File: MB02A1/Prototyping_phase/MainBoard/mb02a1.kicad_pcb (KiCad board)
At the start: 2 copper layers, 7.3 x 1.2 mm, 74 parts, among them J1 USB B mini, J2 USB B mini, J3 USB B mini, J4 USB B mini, U1 CH340G, U11 ACS712-05B, U13 DS1307Z+, U2 CH340G, U3 CH340G, U4 AMS1117-3.3, U5 W25Q64JVS, U6 25LC256, U7 25LC640, U8 NUCLEO-F446RE, U9 WEMOS_D1_mini, X1 12MHz, X2 12MHz, X3 12MHz, X4 32.768 kHz

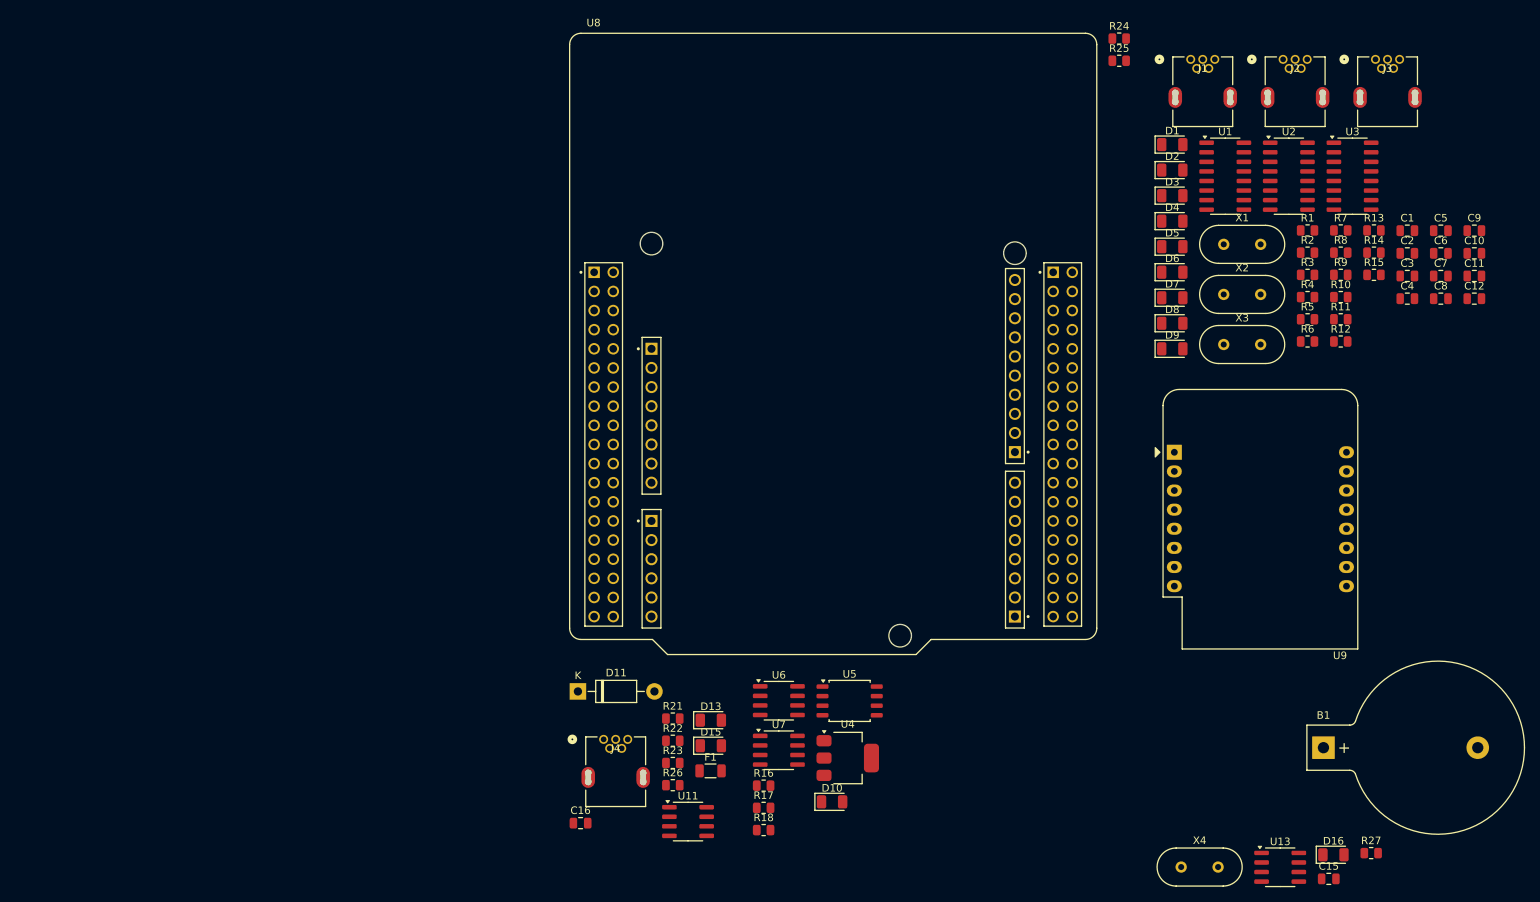
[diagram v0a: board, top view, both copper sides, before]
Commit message: Design update, production preparation.
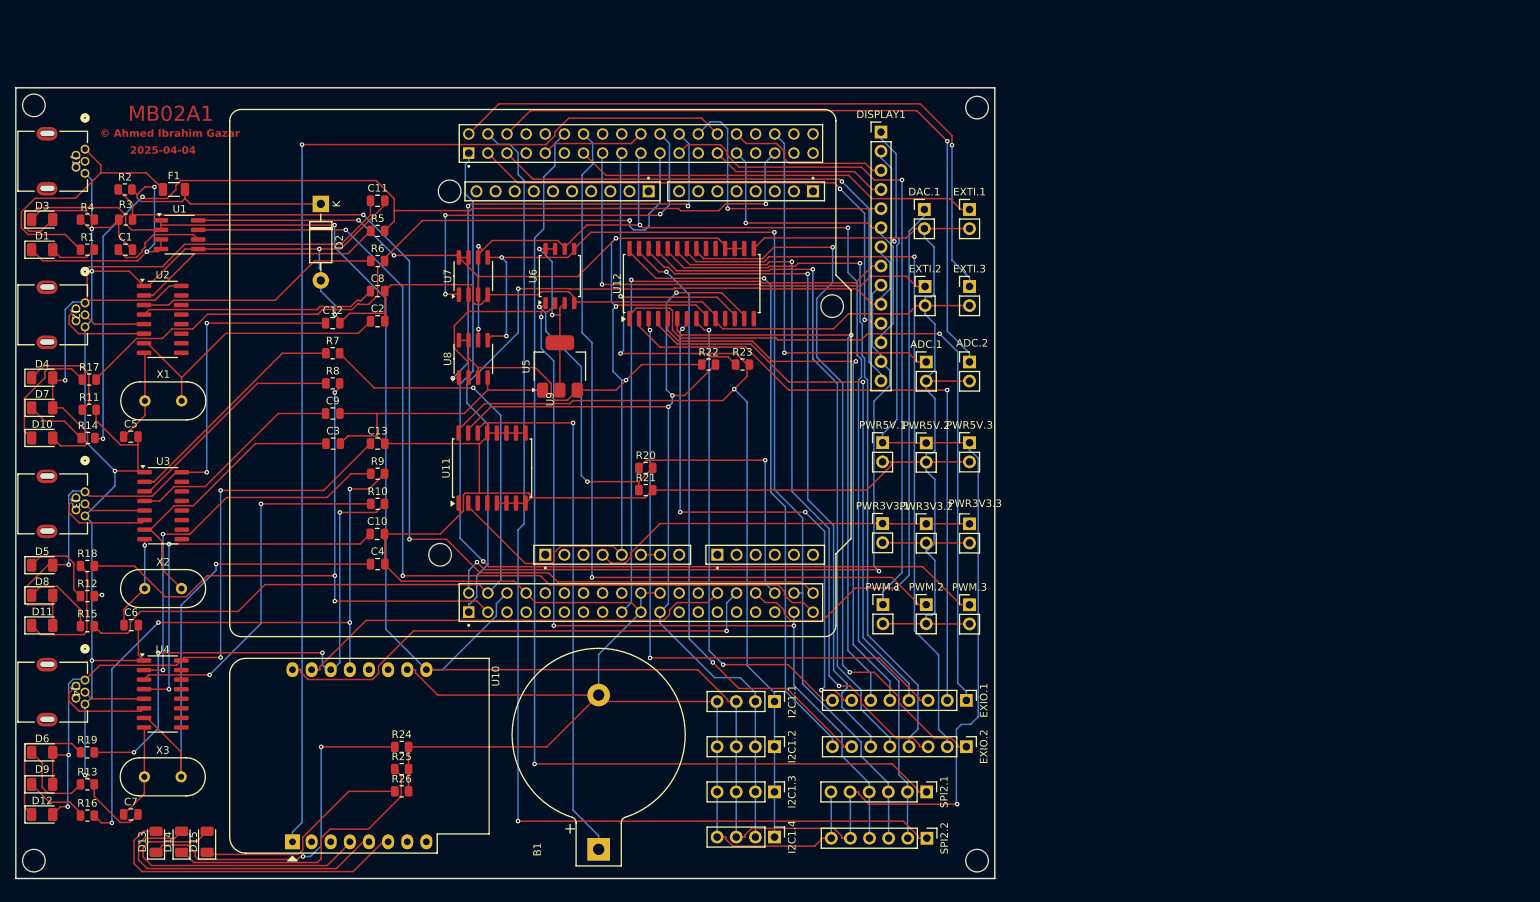
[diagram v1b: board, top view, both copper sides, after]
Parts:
- removed C15: 100p, Capacitor_SMD:C_0805_2012Metric
- removed C16: 1n, Capacitor_SMD:C_0805_2012Metric
- removed D16: D_Schottky, Diode_SMD:D_1206_3216Metric
- removed R27: 1k, Resistor_SMD:R_0805_2012Metric
- removed U13: DS1307Z+, Package_SO:SOIC-8_3.9x4.9mm_P1.27mm
- removed X4: 32.768 kHz, Crystal:Crystal_HC18-U_Vertical
- added ?: , , F.Cu at (80.5, 49.7)
- added ?: , , F.Cu at (80.5, 150.0)
- added ?: , , F.Cu at (205.8, 150.0)
- added ?: , , F.Cu at (205.8, 50.0)
- added ADC.1: Conn_01x02_Pin, Connector_PinHeader_2.54mm:PinHeader_1x02_P2.54mm_Vertical, F.Cu at (199.0, 83.8)
- added ADC.2: Conn_01x02_Pin, Connector_PinHeader_2.54mm:PinHeader_1x02_P2.54mm_Vertical, F.Cu at (204.8, 83.8)
- added C13: 100n, Capacitor_SMD:C_0805_2012Metric, F.Cu at (126.2, 94.6)
- added D12: LED, LED_SMD:LED_1206_3216Metric, F.Cu at (81.6, 143.9)
- added D14: LED, LED_SMD:LED_1206_3216Metric, F.Cu at (100.1, 147.5)
- added DAC.1: Conn_01x02_Pin, Connector_PinHeader_2.54mm:PinHeader_1x02_P2.54mm_Vertical, F.Cu at (198.8, 63.5)
- added DISPLAY1: Conn_01x14_Pin, Connector_PinHeader_2.54mm:PinHeader_1x14_P2.54mm_Vertical, F.Cu at (193.0, 53.3)
- added EXIO.1: Conn_01x08_Pin, Connector_PinHeader_2.54mm:PinHeader_1x08_P2.54mm_Vertical, F.Cu at (204.3, 128.7)
- added EXIO.2: Conn_01x08_Pin, Connector_PinHeader_2.54mm:PinHeader_1x08_P2.54mm_Vertical, F.Cu at (204.3, 134.9)
- added EXTI.1: Conn_01x02_Pin, Connector_PinHeader_2.54mm:PinHeader_1x02_P2.54mm_Vertical, F.Cu at (204.8, 63.5)
- added EXTI.2: Conn_01x02_Pin, Connector_PinHeader_2.54mm:PinHeader_1x02_P2.54mm_Vertical, F.Cu at (198.8, 73.8)
- added EXTI.3: Conn_01x02_Pin, Connector_PinHeader_2.54mm:PinHeader_1x02_P2.54mm_Vertical, F.Cu at (204.8, 73.8)
- added I2C1.1: Conn_01x04_Pin, Connector_PinHeader_2.54mm:PinHeader_1x04_P2.54mm_Vertical, F.Cu at (178.8, 128.9)
- added I2C1.2: Conn_01x04_Pin, Connector_PinHeader_2.54mm:PinHeader_1x04_P2.54mm_Vertical, F.Cu at (178.8, 134.9)
- added I2C1.3: Conn_01x04_Pin, Connector_PinHeader_2.54mm:PinHeader_1x04_P2.54mm_Vertical, F.Cu at (178.8, 140.9)
- added I2C1.4: Conn_01x04_Pin, Connector_PinHeader_2.54mm:PinHeader_1x04_P2.54mm_Vertical, F.Cu at (178.8, 146.9)
- added PWM.1: Conn_01x02_Pin, Connector_PinHeader_2.54mm:PinHeader_1x02_P2.54mm_Vertical, F.Cu at (193.2, 116.0)
- added PWM.2: Conn_01x02_Pin, Connector_PinHeader_2.54mm:PinHeader_1x02_P2.54mm_Vertical, F.Cu at (199.0, 116.0)
- added PWM.3: Conn_01x02_Pin, Connector_PinHeader_2.54mm:PinHeader_1x02_P2.54mm_Vertical, F.Cu at (204.8, 116.0)
- added PWR3V3.1: Conn_01x02_Pin, Connector_PinHeader_2.54mm:PinHeader_1x02_P2.54mm_Vertical, F.Cu at (193.2, 105.2)
- added PWR3V3.2: Conn_01x02_Pin, Connector_PinHeader_2.54mm:PinHeader_1x02_P2.54mm_Vertical, F.Cu at (199.0, 105.3)
- added PWR3V3.3: Conn_01x02_Pin, Connector_PinHeader_2.54mm:PinHeader_1x02_P2.54mm_Vertical, F.Cu at (204.8, 105.3)
- added PWR5V.1: Conn_01x02_Pin, Connector_PinHeader_2.54mm:PinHeader_1x02_P2.54mm_Vertical, F.Cu at (193.2, 94.5)
- added PWR5V.2: Conn_01x02_Pin, Connector_PinHeader_2.54mm:PinHeader_1x02_P2.54mm_Vertical, F.Cu at (199.0, 94.5)
- added PWR5V.3: Conn_01x02_Pin, Connector_PinHeader_2.54mm:PinHeader_1x02_P2.54mm_Vertical, F.Cu at (204.8, 94.5)
- added R19: 1k5, Resistor_SMD:R_0805_2012Metric, F.Cu at (87.6, 135.6)
- added R20: 1k, Resistor_SMD:R_0805_2012Metric, F.Cu at (161.8, 97.8)
- added SPI2.1: Conn_01x06_Pin, Connector_PinHeader_2.54mm:PinHeader_1x06_P2.54mm_Vertical, F.Cu at (199.1, 140.9)
- added SPI2.2: Conn_01x06_Pin, Connector_PinHeader_2.54mm:PinHeader_1x06_P2.54mm_Vertical, F.Cu at (199.1, 147.0)
- added U10: WEMOS_D1_mini, RF_Module:WEMOS_D1_mini_light, F.Cu at (114.8, 147.5)
- added U12: MCP23017_SO, Package_SO:SOIC-28W_7.5x17.9mm_P1.27mm, F.Cu at (167.8, 73.4)
- C1: value 22p -> 1n
- C10, C9: value 22p -> 100n
- C3, C4, C7: value 100n -> 22p
- D11: value 1N4001 -> LED; footprint Diode_THT:D_DO-41_SOD81_P10.16mm_Horizontal -> LED_SMD:LED_1206_3216Metric
- D2: value LED -> 1N4001; footprint LED_SMD:LED_1206_3216Metric -> Diode_THT:D_DO-41_SOD81_P10.16mm_Horizontal
- R1: value 1k5 -> 220R
- R17: value 1k -> 1k5
- R18: value 2k -> 1k5
- R2, R3: value 1k5 -> 10k
- R21: value 220R -> 2k
- R22, R23: value 10k -> 4k7
- R24, R25: value 4k7 -> 1k5
- U1: value CH340G -> ACS712-05B; footprint Package_SO:SOIC-16_3.9x9.9mm_P1.27mm -> Package_SO:SOIC-8_3.9x4.9mm_P1.27mm
- U11: value ACS712-05B -> DS3231M; footprint Package_SO:SOIC-8_3.9x4.9mm_P1.27mm -> Package_SO:SOIC-16W_7.5x10.3mm_P1.27mm
- U4: value AMS1117-3.3 -> CH340G; footprint Package_TO_SOT_SMD:SOT-223-3_TabPin2 -> Package_SO:SOIC-16_3.9x9.9mm_P1.27mm
- U5: value W25Q64JVS -> AMS1117-3.3; footprint Package_SO:SOIC-8_5.23x5.23mm_P1.27mm -> Package_TO_SOT_SMD:SOT-223-3_TabPin2
- U6: value 25LC256 -> W25Q64JVS; footprint Package_SO:SOIC-8_3.9x4.9mm_P1.27mm -> Package_SO:SOIC-8_5.23x5.23mm_P1.27mm
- U7: value 25LC640 -> 25LC256
- U8: value NUCLEO-F446RE -> 25LC640; footprint NUCLEO-F446RE:MODULE_NUCLEO-F446RE -> Package_SO:SOIC-8_3.9x4.9mm_P1.27mm
- U9: value WEMOS_D1_mini -> NUCLEO-F446RE; footprint RF_Module:WEMOS_D1_mini_light -> NUCLEO-F446RE:MODULE_NUCLEO-F446RE
- X1, X2, X3: value 12MHz -> 12 MHz; footprint Crystal:Crystal_HC18-U_Vertical -> Crystal:Crystal_HC49-U_Vertical
- moved C7 188.1 mm to (93.4, 143.9)
- moved R13 186.0 mm to (87.6, 139.9)
- moved C6 180.8 mm to (93.4, 118.7)
- moved J3 180.7 mm to (87.3, 101.0), turned to -90 degrees
- moved R15 177.1 mm to (87.6, 118.9)
- moved C5 176.1 mm to (93.4, 93.7)
- moved R14 172.5 mm to (87.7, 93.9)
- moved C1 170.3 mm to (92.7, 68.9)
- moved R12 169.8 mm to (87.6, 114.9)
- moved R11 166.6 mm to (87.8, 90.1)
- moved U3 163.9 mm to (97.7, 102.9)
- moved D6 163.1 mm to (81.6, 135.6)
- moved R4 162.4 mm to (87.6, 64.9)
- moved J2 162.4 mm to (87.3, 75.9), turned to -90 degrees
- moved R1 162.1 mm to (87.6, 68.9)
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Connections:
- B1 pad 1: Net-(D16-A) -> Net-(U11-VBAT)
- C1 pad 1: Net-(U1-XI) -> Net-(U1-FILTER)
- C10 pad 1: Net-(U3-XO) -> Net-(U4-V3)
- C11 pad 1: Net-(U3-V3) -> VBUS1
- C12 pad 1: VBUS3 -> VBUS2
- C2 pad 1: Net-(U1-XO) -> Net-(U2-XI)
- C3 pad 1: Net-(U1-V3) -> Net-(U3-XI)
- C4 pad 1: VBUS1 -> Net-(U4-XI)
- C5 pad 1: Net-(U2-XI) -> Net-(U2-XO)
- C6 pad 1: Net-(U2-XO) -> Net-(U3-XO)
- C7 pad 1: Net-(U2-V3) -> Net-(U4-XO)
- C8 pad 1: VBUS2 -> Net-(U2-V3)
- C9 pad 1: Net-(U3-XI) -> Net-(U3-V3)
- D1 pad 2: VBUS1 -> Net-(D1-A)
- D10 pad 2: M5V -> VBUS1
- D11 pad 2: GND -> VBUS2
- D13 pad 1: Net-(D11-K) -> Net-(D13-K)
- D15 pad 2: 5V_REG -> Net-(D15-A)
- D2 pad 1: Net-(D2-K) -> Net-(D1-K)
- D2 pad 2: VBUS1 -> GND
- D3 pad 2: VBUS1 -> 5V_REG
- D4 pad 2: VBUS2 -> VBUS1
- D6 pad 2: VBUS2 -> VBUS3
- D7 pad 2: VBUS3 -> VBUS1
- D8 pad 2: VBUS3 -> VBUS2
- F1 pad 1: Net-(J4-VBUS) -> Net-(J1-VBUS)
- F1 pad 2: Net-(D11-K) -> Net-(D1-K)
- J1 pad 1: VBUS1 -> Net-(J1-VBUS)
- J1 pad 2: D1- -> unconnected-(J1-D--Pad2)
- J1 pad 3: D1+ -> unconnected-(J1-D+-Pad3)
- J2 pad 1: VBUS2 -> VBUS1
- J2 pad 2: D2- -> D1-
- J2 pad 3: D2+ -> D1+
- J3 pad 1: VBUS3 -> VBUS2
- J3 pad 2: D3- -> D2-
- J3 pad 3: D3+ -> D2+
- J4 pad 1: Net-(J4-VBUS) -> VBUS3
- J4 pad 2: unconnected-(J4-D--Pad2) -> D3-
- J4 pad 3: unconnected-(J4-D+-Pad3) -> D3+
- R1 pad 1: Net-(U1-TXD) -> Net-(J1-VBUS)
- R1 pad 2: USART1_RX -> Net-(D1-A)
- R10 pad 1: Net-(D6-K) -> Net-(U4-RXD)
- R10 pad 2: UART5_TX -> WUART1_TX
- R11 pad 1: Net-(U3-TXD) -> Net-(D4-K)
- R11 pad 2: WUART1_RX -> GND
- R12 pad 1: Net-(U3-RXD) -> Net-(D5-K)
- R12 pad 2: WUART1_TX -> GND
- R13 pad 1: Net-(D7-K) -> Net-(D6-K)
- R14 pad 1: Net-(D8-K) -> Net-(D7-K)
- R14 pad 2: WUART1_RX -> USART1_RX
- R15 pad 1: Net-(D9-K) -> Net-(D8-K)
- R15 pad 2: WUART1_TX -> UART5_RX
- R16 pad 1: Net-(D10-K) -> Net-(D9-K)
- R16 pad 2: GND -> WUART1_RX
- R17 pad 1: W25Q64_NCS -> Net-(D10-K)
- R17 pad 2: W25Q64_NCS3V3 -> USART1_TX
- R18 pad 1: W25Q64_NCS3V3 -> Net-(D11-K)
- R18 pad 2: GND -> UART5_TX
- R2 pad 1: Net-(U1-RXD) -> U_PWR_MEAS
- R2 pad 2: USART1_TX -> Net-(D1-K)
- R21 pad 1: Net-(J4-VBUS) -> W25Q64_NCS3V3
- R21 pad 2: Net-(D13-A) -> GND
- R22 pad 1: U_PWR_MEAS -> M5V
- R22 pad 2: Net-(D11-K) -> I2C1_SDA
- R23 pad 1: GND -> M5V
- R23 pad 2: U_PWR_MEAS -> I2C1_SCL
- R24 pad 1: M5V -> Net-(D13-K)
- R24 pad 2: I2C1_SDA -> GND
- R25 pad 1: M5V -> Net-(D14-K)
- R25 pad 2: I2C1_SCL -> GND
- R26 pad 1: GND -> Net-(D15-K)
- R26 pad 2: Net-(D15-K) -> GND
- R3 pad 1: Net-(D1-K) -> GND
- R3 pad 2: GND -> U_PWR_MEAS
- R4 pad 1: Net-(D2-K) -> GND
- R4 pad 2: USART1_RX -> Net-(D3-K)
- R5 pad 1: Net-(D3-K) -> Net-(U2-TXD)
- R5 pad 2: USART1_TX -> USART1_RX
- R6 pad 1: Net-(U2-TXD) -> Net-(U2-RXD)
- R6 pad 2: UART5_RX -> USART1_TX
- R7 pad 1: Net-(U2-RXD) -> Net-(U3-TXD)
- R7 pad 2: UART5_TX -> UART5_RX
- R8 pad 1: Net-(D4-K) -> Net-(U3-RXD)
- R8 pad 2: GND -> UART5_TX
- R9 pad 1: Net-(D5-K) -> Net-(U4-TXD)
- R9 pad 2: UART5_RX -> WUART1_RX
- U1 pad 1: GND -> 5V_REG
- U1 pad 2: Net-(U1-TXD) -> 5V_REG
- U1 pad 3: Net-(U1-RXD) -> Net-(D1-K)
- U1 pad 4: Net-(U1-V3) -> Net-(D1-K)
- U1 pad 5: D1+ -> GND
- U1 pad 6: D1- -> Net-(U1-FILTER)
- U1 pad 7: Net-(U1-XI) -> I_PWR_MEAS
- U1 pad 8: Net-(U1-XO) -> M5V
- U11 pad 1: 5V_REG -> unconnected-(U11-32KHZ-Pad1)
- U11 pad 2: 5V_REG -> M5V
- U11 pad 3: Net-(D11-K) -> unconnected-(U11-~{INT}/SQW-Pad3)
- U11 pad 4: Net-(D11-K) -> unconnected-(U11-~{RST}-Pad4)
- U11 pad 6: Net-(U11-FILTER) -> GND
- U11 pad 7: I_PWR_MEAS -> GND
- U11 pad 8: M5V -> GND
- U2 pad 16: VBUS2 -> VBUS1
- U2 pad 5: D2+ -> D1+
- U2 pad 6: D2- -> D1-
- U3 pad 16: VBUS3 -> VBUS2
- U3 pad 5: D3+ -> D2+
- U3 pad 6: D3- -> D2-
- U4 pad 2: Net-(U4-VO) -> Net-(U4-TXD)
- U4 pad 3: M5V -> Net-(U4-RXD)
- U5 pad 1: W25Q64_NCS3V3 -> GND
- U5 pad 2: SPI2_MISO -> Net-(U5-VO)
- U5 pad 3: Net-(U4-VO) -> M5V
- U6 pad 1: 25LC256_NCS -> W25Q64_NCS3V3
- U6 pad 3: M5V -> Net-(U5-VO)
- U6 pad 7: M5V -> Net-(U5-VO)
- U6 pad 8: M5V -> Net-(U5-VO)
- U7 pad 1: 25LC640_NCS -> 25LC256_NCS
- X1 pad 1: Net-(U1-XO) -> Net-(U2-XO)
- X1 pad 2: Net-(U1-XI) -> Net-(U2-XI)
- X2 pad 1: Net-(U2-XO) -> Net-(U3-XO)
- X2 pad 2: Net-(U2-XI) -> Net-(U3-XI)
- X3 pad 1: Net-(U3-XO) -> Net-(U4-XO)
- X3 pad 2: Net-(U3-XI) -> Net-(U4-XI)
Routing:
- net GND: track 0.00 -> 753.6 mm, vias 0 -> 9
- net 5V_REG: track 0.00 -> 335.2 mm, vias 0 -> 2
- net M5V: track 0.00 -> 212.2 mm, vias 0 -> 5
- net I2C1_SCL: track 0.00 -> 166.4 mm, vias 0 -> 3
- net SPI2_SCK: track 0.00 -> 159.9 mm, vias 0 -> 4
- net WEMOS_RST: track 0.00 -> 150.9 mm, vias 0 -> 1
- net SPI2_CS1: track 0.00 -> 149.9 mm, vias 0 -> 1
- net SPI2_MOSI: track 0.00 -> 141.0 mm, vias 0 -> 3
- net SPI2_CS0: track 0.00 -> 139.1 mm, vias 0 -> 1
- net U_PWR_MEAS: track 0.00 -> 137.6 mm, vias 0 -> 2
- net USART1_RX: track 0.00 -> 133.4 mm, vias 0 -> 3
- net SPI2_MISO: track 0.00 -> 133.1 mm, vias 0 -> 3
- net I2C1_SDA: track 0.00 -> 128.3 mm, vias 0 -> 3
- net I_PWR_MEAS: track 0.00 -> 125.4 mm, vias 0 -> 2
- net PWM3: track 0.00 -> 123.8 mm, vias 0 -> 1
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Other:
- board size 7.3 x 1.2 mm -> 130 x 105 mm
- board text added: "2025-04-04"
- board text added: "MB02A1"
- board text added: "© Ahmed Ibrahim Gazar"
